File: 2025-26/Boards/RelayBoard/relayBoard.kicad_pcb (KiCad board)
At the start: 2 copper layers, 53.5 x 71.2 mm, 70 parts, among them J1 043045-1212, J2 Conn_01x04_Pin, K4 HF42F/012-2HST, K5 HF42F/012-2HST, K6 HF42F/012-2HST, K7 HF42F/012-2HST, Q1 AO3400A, Q10 AO3400A, Q11 AO3400A, Q2 AO3400A, Q3 AO3401A, Q4 AO3400A, Q5 AO3400A, Q6 AO3401A, Q7 AO3400A, Q9 AO3400A, U4 UA78M33QDCYRQ1, U5 STM32C011F4Px

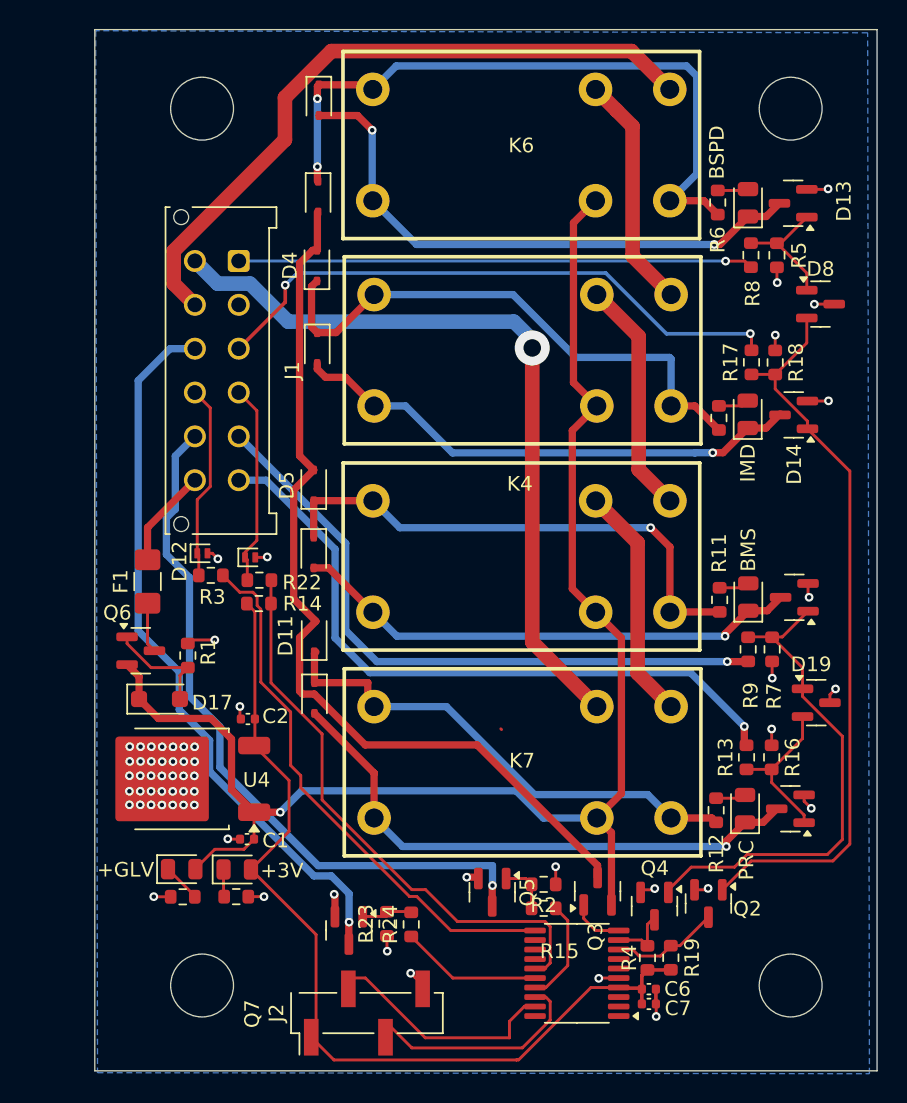
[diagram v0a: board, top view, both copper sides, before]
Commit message: relay board revision
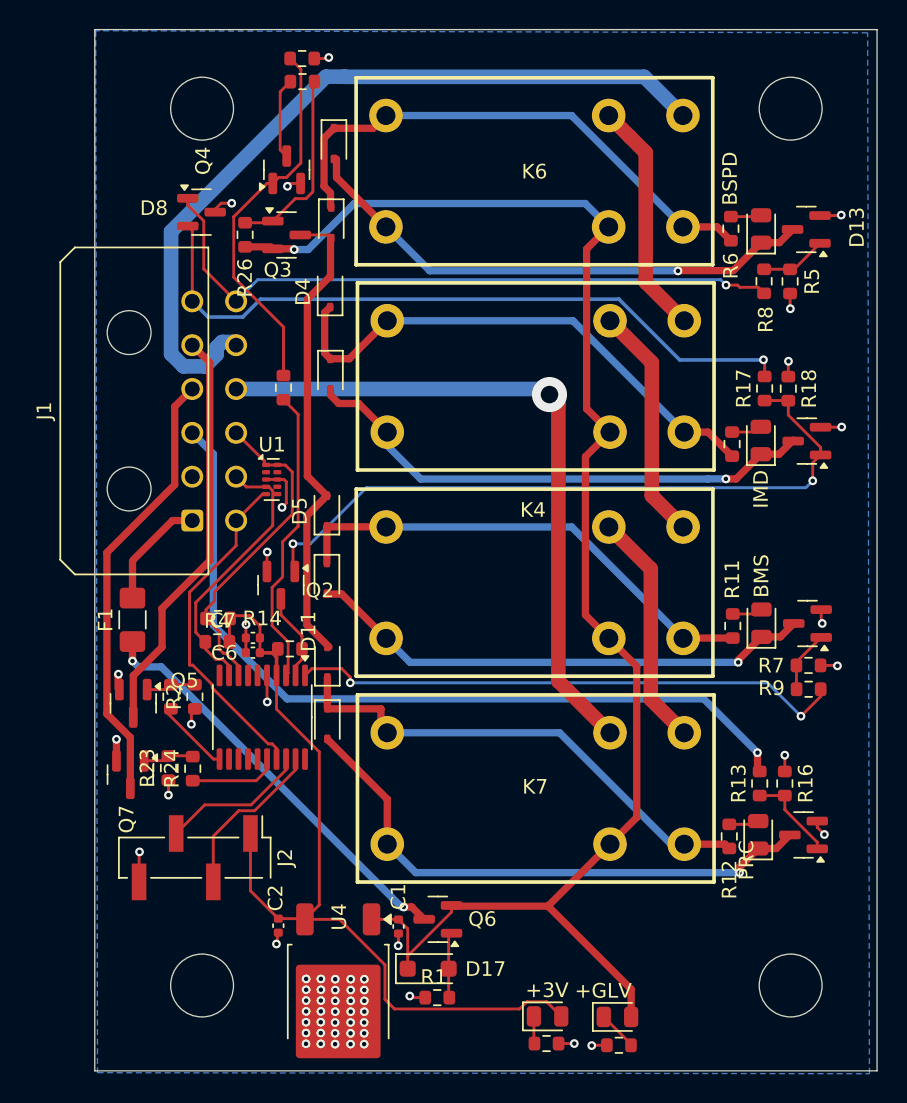
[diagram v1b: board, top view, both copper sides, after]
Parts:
- removed D12, D7: PESD5V0S1UL, Diode_SMD:D_SOD-882
- removed D19: PSM712-LF-T7, Package_TO_SOT_SMD:SOT-23
- removed R3: 330, Resistor_SMD:R_0603_1608Metric
- added R25: 47, Resistor_SMD:R_0603_1608Metric, F.Cu at (93.0, 37.1)
- added R26: 100k, Resistor_SMD:R_0603_1608Metric, F.Cu at (89.1, 47.6)
- added R27: 100k, Resistor_SMD:R_0603_1608Metric, F.Cu at (93.0, 35.5)
- added U1: TPD4E05U06DQA, Package_SON:USON-10_2.5x1.0mm_P0.5mm, F.Cu at (90.9, 64.3)
- J1: footprint Connector_Molex:Molex_Micro-Fit_3.0_43045-1212_2x06_P3.00mm_Vertical -> Connector_Molex:Molex_Micro-Fit_3.0_43045-1200_2x06_P3.00mm_Horizontal
- Q3: value AO3401A -> AO3407A
- R1: value R -> 13k
- R22: value 330 -> 47
- R7: value 12k -> 100k
- R9: value 3k -> 47
- moved Q4 56.3 mm to (92.0, 43.1), turned to 90 degrees
- moved Q3 49.7 mm to (91.9, 47.6), turned to 0 degrees
- moved D8 42.8 mm to (86.1, 46.0)
- moved C7 36.9 mm to (89.6, 75.1), turned to 180 degrees
- moved R4 36.5 mm to (87.2, 75.4), turned to 0 degrees
- moved Q2 36.5 mm to (91.6, 71.5)
- moved C6 35.5 mm to (89.6, 76.2), turned to 0 degrees
- moved R19 33.5 mm to (92.2, 75.9), turned to 0 degrees
- moved R21 31.5 mm to (114.7, 103.0)
- moved GLV1 31.5 mm to (114.6, 101.1)
- moved R15 29.3 mm to (84.0, 79.2), turned to 90 degrees
- moved R1 29.0 mm to (102.2, 99.8), turned to 180 degrees
- moved Q5 27.8 mm to (81.5, 79.6)
- moved U5 27.8 mm to (90.3, 80.6), turned to -90 degrees
- moved Q6 27.4 mm to (102.3, 94.4), turned to 180 degrees
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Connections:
- net +12V renamed GLV+
- net Precharge_gate renamed Net-(Q11-G)
- D8 pad 1: BSPD_gate -> BSPD Fault
- D8 pad 2: IMD_Gate -> IMD Fault
- J1 pad 1: BSPD Fault -> BAT+
- J1 pad 10: No_Faults -> SDC 2
- J1 pad 11: Extra_GPIO1 -> SDC 1
- J1 pad 12: BAT+ -> BSPD Fault
- J1 pad 3: IMD Fault -> Precharge_fault
- J1 pad 4: Reset -> Extra_GPIO2
- J1 pad 5: BMS Fault -> Extra_GPIO1
- J1 pad 6: Precharge_fault -> IMD Fault
- J1 pad 7: SDC 2 -> No_Faults
- J1 pad 8: SDC 1 -> BMS Fault
- J1 pad 9: Extra_GPIO2 -> Reset
- Q10 pad 1: BMS_gate -> Net-(Q10-G)
- Q3 pad 1: Reset_Latch -> Net-(Q3-G)
- Q4 pad 1: BMS_gate -> Net-(Q4-G)
- R14 pad 1: Net-(U5-PA8) -> Reset
- R15 pad 1: Net-(U5-PA10/PA12) -> Net-(U5-PA4)
- R22 pad 1: Reset -> Reset_Latch
- R22 pad 2: Net-(U5-PA8) -> Net-(Q4-G)
- R4 pad 1: +3.3V -> BMS Fault
- R4 pad 2: Net-(Q4-D) -> +3.3V
- R7 pad 2: BMS_gate -> Net-(Q10-G)
- R9 pad 1: BMS_gate -> Net-(Q10-G)
- R9 pad 2: BMS Fault -> BMS_Gate
- U5 pad 1: unconnected-(U5-PB7-Pad1) -> BMS_Gate
- U5 pad 10: Reset_Latch -> unconnected-(U5-PA3-Pad10)
- U5 pad 15: Net-(U5-PA8) -> unconnected-(U5-PA8-Pad15)
- U5 pad 17: Net-(U5-PA10/PA12) -> No_Faults
- U5 pad 2: unconnected-(U5-PC14-Pad2) -> Net-(Q2-D)
- U5 pad 3: unconnected-(U5-PC15-Pad3) -> Reset_Latch
- U5 pad 8: Net-(Q2-D) -> Reset
- U5 pad 9: Net-(Q4-D) -> BMS Fault
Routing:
- net Net-(U5-PA8): track 40.1 -> 0.00 mm
- net BMS_Gate: track 0.00 -> 38.1 mm, vias 0 -> 2
- net BMS_gate: track 33.8 -> 0.00 mm
- net Net-(U5-PA4): track 37.4 -> 5.12 mm
- net Net-(D11-A): track 61.7 -> 32.7 mm
- net Net-(Q4-G): track 0.00 -> 25.8 mm
- net BMS Fault: track 44.7 -> 18.9 mm, vias 1 -> 0
- net Net-(Q6-D): track 3.44 -> 28.3 mm, vias 0 -> 2
- net Extra_GPIO1: track 48.8 -> 28.1 mm, vias 1 -> 0
- net Extra_GPIO2: track 50.0 -> 30.4 mm, vias 1 -> 0
- net Reset_Latch: track 3.67 -> 20.5 mm
- net Net-(Q3-G): track 0.00 -> 12.9 mm
- net BSPD Fault: track 35.2 -> 45.5 mm
- net No_Faults: track 13.4 -> 23.1 mm
- net Precharge_fault: track 46.5 -> 55.9 mm
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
